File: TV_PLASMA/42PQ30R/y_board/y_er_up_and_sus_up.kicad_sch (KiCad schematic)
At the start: 43 parts, among them Q11 Q_NIGBT_GCE, Q12 Q_NIGBT_GCE, Q13 Q_NIGBT_GCE, Q14 Q_NIGBT_GCE, Q701 Q_NPN_BCE, Q702 Q_PNP_BCE

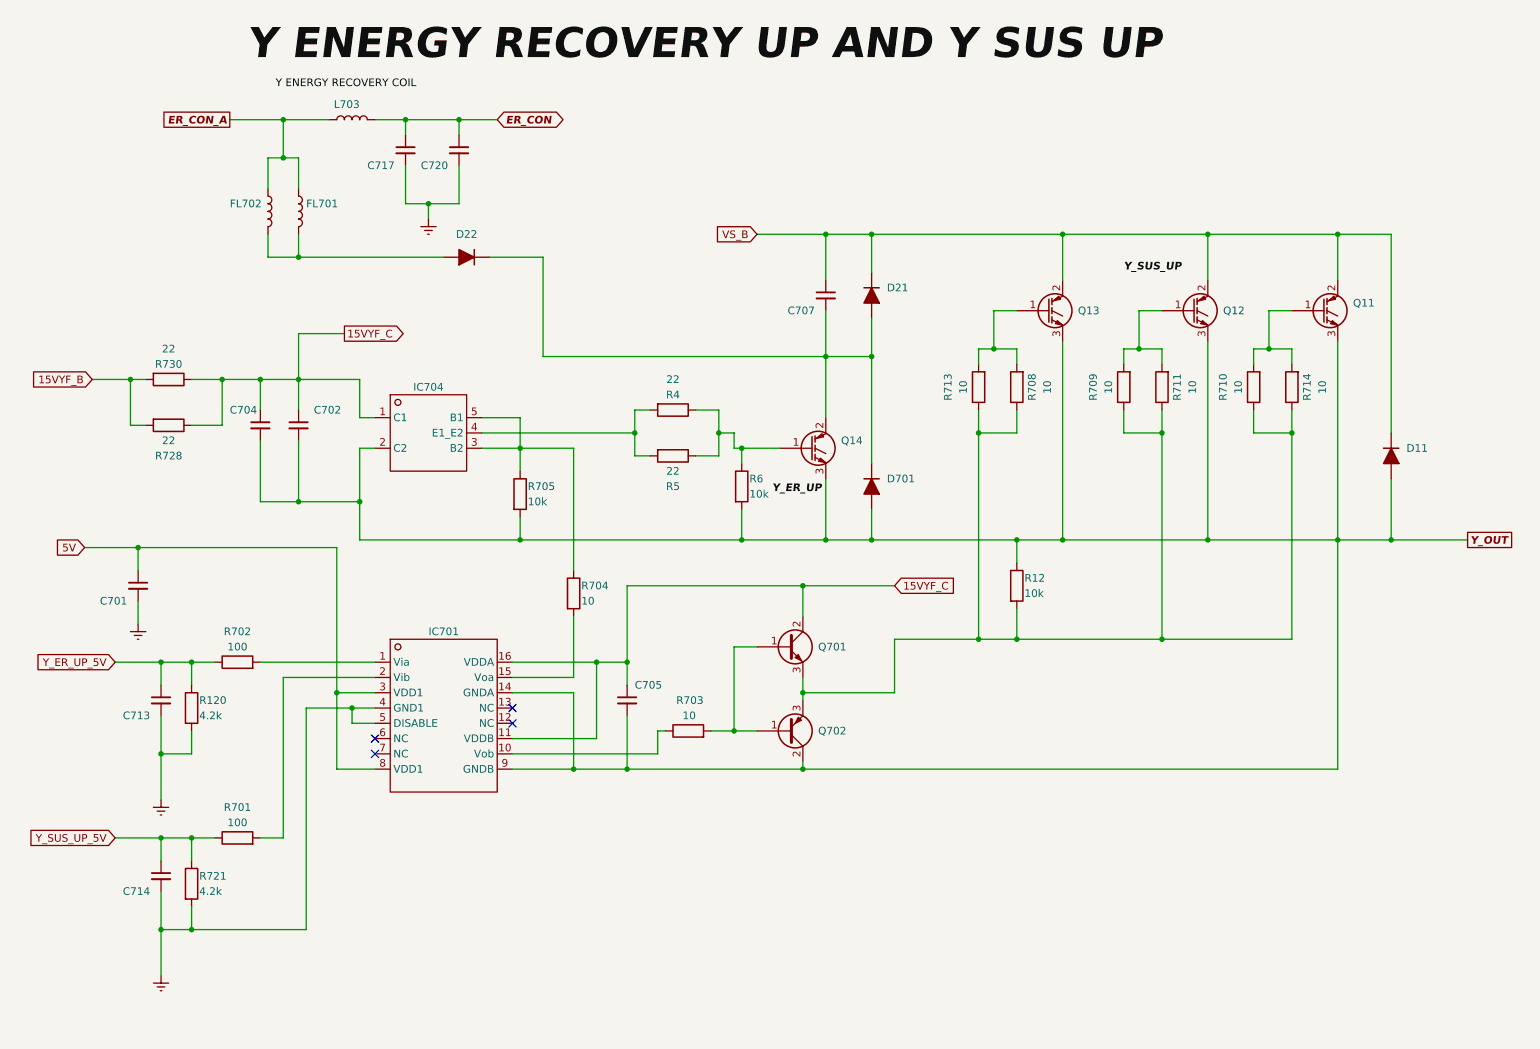
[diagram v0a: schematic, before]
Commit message: Finishing 15VF, 5VF and 15V power supply
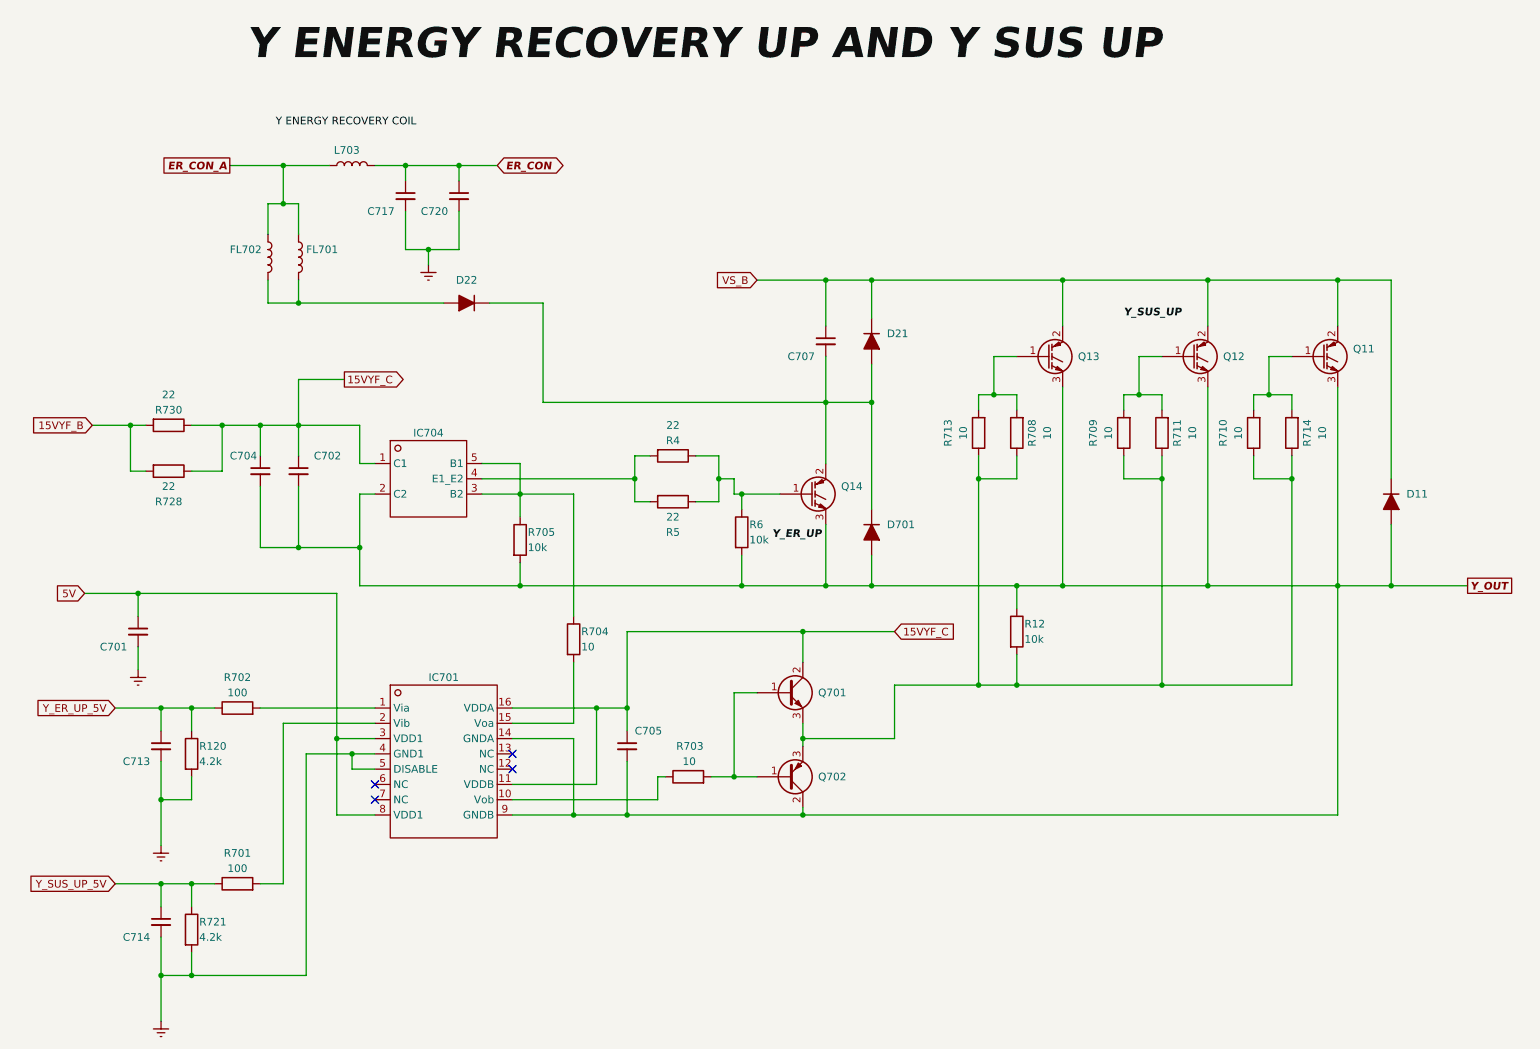
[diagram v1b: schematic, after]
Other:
- moved on the sheet: C701, C702, C704, C705, C707, C713, C714, C717, C720, D11, D21, D22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
